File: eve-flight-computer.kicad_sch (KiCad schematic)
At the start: 0 parts

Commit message: Rev. 1
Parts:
- added BT1: ML414H, kicad-egglib:ML414H, symbol Device:Battery_Cell
- added C1, C26: 4.7uF, kicad-egglib:0402_1005M, symbol Device:C_Small
- added C10, C11, C12, C13, C14, C15, C17, C2, C21, C22, C23, C24, C25, C27, C28, C29, C3, C30, C31, C33, C34, C36, C37, C4, C42, C5, C54, C6, C7, C8, C9: 100nF, kicad-egglib:0402_1005M, symbol Device:C_Small
- added C16, C18: 2.2uF, kicad-egglib:0402_1005M, symbol Device:C_Small
- added C19, C32, C35, C43, C44, C45: 10uF, kicad-egglib:0805_2012M, symbol Device:C_Small
- added C20, C38, C39, C40, C41, C46, C47, C48, C49, C50, C51: 47uF, Capacitor_SMD:C_1206_3216Metric, symbol Device:C_Small
- added C52, C53: 22uF, kicad-egglib:0805_2012M, symbol Device:C_Small
- added D1: Red, Diode_SMD:D_0603_1608Metric, symbol Device:LED_Small
- added D10, D11, D6, D9: 11V, Diode_SMD:D_SOD-123, symbol Device:D_Zener_Small
- added D2: Green, Diode_SMD:D_0603_1608Metric, symbol Device:LED_Small
- added D3: Blue, Diode_SMD:D_0603_1608Metric, symbol Device:LED_Small
- added D4: Yellow, Diode_SMD:D_0603_1608Metric, symbol Device:LED_Small
- added D5: PMEG4005EJ, Diode_SMD:D_SOD-323, symbol Device:D_Small
- added D7, D8: UPS115UE3, Diode_SMD:D_Powermite_AK, symbol Device:D_Small
- added J1: USB4110, Connector_USB:USB_C_Receptacle_GCT_USB4110, symbol kicad-egglib:USB-C-2
- added J10, J11, J13, J14, J8, J9: SERVO, Connector_PinHeader_2.54mm:PinHeader_1x03_P2.54mm_Vertical, symbol Connector:Conn_01x03_Pin
- added J12: PYRO, Connector_PinSocket_2.54mm:PinSocket_1x12_P2.54mm_Vertical, symbol Connector:Conn_01x12_Socket
- added J2: ARM Cortex Debug, Connector_PinHeader_1.27mm:PinHeader_2x05_P1.27mm_Vertical_SMD, symbol kicad-egglib:ARM_Cortex_Debug
- added J3: GPIO, Connector_PinSocket_2.54mm:PinSocket_1x12_P2.54mm_Vertical, symbol Connector:Conn_01x12_Socket
- added J4, J5, J6: SMA, Connector_Coaxial:SMA_Amphenol_132289_EdgeMount, symbol Connector:Conn_Coaxial
- added J7: XT-60, kicad-egglib:XT60PW-M, symbol Connector:Conn_01x02_Socket
- added JP1: VSEL, Jumper:SolderJumper-3_P1.3mm_Open_Pad1.0x1.5mm, symbol Jumper:SolderJumper_3_Open
- added L1: 4.7uH, Inductor_SMD:L_1210_3225Metric, symbol Device:L_Small
- added Q1, Q10, Q2, Q3, Q4, Q5, Q6, Q7, Q8: DMG3402L, Package_TO_SOT_SMD:SOT-23-3, symbol Device:Q_NMOS_GSD
- added Q11, Q9: DMP3099L, Package_TO_SOT_SMD:SOT-23-3, symbol Device:Q_PMOS_GSD
- added R1, R2: 5.1k, kicad-egglib:0402_1005M, symbol Device:R_Small_US
- added R10, R30: 3.3k, kicad-egglib:0402_1005M, symbol Device:R_Small_US
- added R11, R12, R13, R14, R15, R16, R17, R20, R4: 100k, kicad-egglib:0402_1005M, symbol Device:R_Small_US
- added R18, R19, R22, R27, R28, R29, R34, R38, R6, R7, R8, R9: 1k, kicad-egglib:0402_1005M, symbol Device:R_Small_US
- added R21, R23, R24, R25, R26, R31, R32, R33, R35, R36, R37, R39, R40, R41, R42, R43, R44: 10k, kicad-egglib:0402_1005M, symbol Device:R_Small_US
- added R3: 33k, kicad-egglib:0402_1005M, symbol Device:R_Small_US
- added R5: 82k, kicad-egglib:0402_1005M, symbol Device:R_Small_US
- added U1: USBLC6-2SC6, Package_TO_SOT_SMD:SOT-23-6, symbol kicad-egglib:USBLC6-2SC6
- added U10: MLX90395KDC, Package_SO:SOIC-8_3.9x4.9mm_P1.27mm, symbol kicad-egglib:MLX90395KDC
- added U11, U8: W25N01GVZEIG, Package_SON:WSON-8-1EP_8x6mm_P1.27mm_EP3.4x4.3mm, symbol kicad-egglib:W25N01GVZEIx
- added U12: LDL1117, Package_TO_SOT_SMD:SOT-223-3_TabPin2, symbol kicad-egglib:Generic_Regulator_GroundOutputInput
- added U13: AP62200WU, Package_TO_SOT_SMD:SOT-23-6, symbol kicad-egglib:AP62200WU
- added U14: INA260, Package_SO:TSSOP-16_4.4x5mm_P0.65mm, symbol kicad-egglib:INA260
- added U15, U16, U17, U18, U19, U20: SN74LVC1T45DBV, Package_TO_SOT_SMD:SOT-23-6, symbol kicad-egglib:SN74LVC1T45DBV
- added U2: STM32H733ZGT6, Package_QFP:LQFP-144_20x20mm_P0.5mm, symbol kicad-egglib:STM32F765ZxTx
- added U3: BMI088, kicad-egglib:BMI088, symbol kicad-egglib:BMI088
- added U4: H3LIS331DL, Package_LGA:LGA-16_3x3mm_P0.5mm_LayoutBorder3x5y, symbol kicad-egglib:H3LIS331DL
- added U5: RFM95W-915S2, kicad-egglib:RFM9xW-xxxS2, symbol kicad-egglib:RFM9xW-xxxS2
- added U6: ZOE-M8Q, kicad-egglib:ZOE-M8Q, symbol kicad-egglib:ZOE-M8Q
- added U7: MS560702BA03-50, kicad-egglib:MS5607-02BA, symbol kicad-egglib:MS5607-02BA
- added U9: RFM96W-433S2, kicad-egglib:RFM9xW-xxxS2, symbol kicad-egglib:RFM9xW-xxxS2
- added Y1: 48MHz, Crystal:Crystal_SMD_2520-4Pin_2.5x2.0mm, symbol Device:Crystal_GND24_Small
- added Y2: 32.768kHz, Crystal:Crystal_SMD_MicroCrystal_CM9V-T1A-2Pin_1.6x1.0mm, symbol Device:Crystal_Small
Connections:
- new net: J12.4 (Pin_4), Q4.3 (D), R27.1
- new net: D9.1 (K), Q3.1 (G), R27.2, R31.1
- new net: C42.2, L1.1, U13.2 (SW)
- new net: C45.1, D7.1 (K), D8.1 (K), U13.3 (VIN)
- new net: R26.2, R30.1, U13.4 (FB)
- new net: C42.1, U13.6 (BST)
- new net: D11.1 (K), Q7.1 (G), R38.2, R39.1
- new net: C44.1, JP1.1 (A), U12.2 (VOUT)
- new net: J12.11 (Pin_11), J7.1 (Pin_1), U14.1 (IN+), U14.12 (VBUS), U14.2 (IN+), U14.3 (IN+)
- new net: J1.A5 (CC1), R2.1
- new net: J12.8 (Pin_8), Q8.3 (D), R38.1
- new net: D6.1 (K), Q1.1 (G), R22.2, R23.1
- new net: J4.1 (In), U6.A4 (RF_IN)
- new net: BT1.1 (+), C25.1, C26.1, R10.1, U6.H9 (V_BCKP)
- new net: U6.J7 (RTC_I), Y2.2
- new net: U6.J8 (RTC_O), Y2.1
- new net: J12.6 (Pin_6), Q6.3 (D), R34.1
- new net: J9.3 (Pin_3), U16.4 (B)
- new net: J6.1 (In), U9.9 (ANT)
- new net: J1.A7 (D-), J1.B7 (D-), U1.4
- new net: J1.A6 (D+), J1.B6 (D+), U1.6
- new net: D10.1 (K), Q5.1 (G), R34.2, R35.1
- new net: Q10.1 (G), Q11.3 (D), R42.1
- new net: J13.3 (Pin_3), U19.4 (B)
- new net: JP1.2 (C), U15.6 (VCCB), U16.6 (VCCB), U17.6 (VCCB), U18.6 (VCCB), U19.6 (VCCB), U20.6 (VCCB)
- new net: D4.2 (A), R9.2
- new net: U2.23 (PH0), Y1.3
- new net: R3.2, R5.1, U2.101 (PA9)
- new net: J1.B5 (CC2), R1.1
- new net: C16.1, U2.71 (VCAP1)
- new net: C18.1, U2.106 (VCAP2)
- new net: J14.3 (Pin_3), U20.4 (B)
- new net: J5.1 (In), U5.9 (ANT)
- new net: Q10.3 (D), Q9.1 (G), R40.2
- new net: D3.2 (A), R8.2
- new net: D2.2 (A), R7.2
- new net: J11.3 (Pin_3), U18.4 (B)
- new net: J12.2 (Pin_2), Q2.3 (D), R22.1
- new net: J8.3 (Pin_3), U15.4 (B)
- new net: D1.2 (A), R6.2
- new net: D5.1 (K), R10.2
- new net: J10.3 (Pin_3), U17.4 (B)
- new net +3.3V: C1.1, C10.1, C11.1, C12.1, C13.1, C14.1, C15.1, C19.1, C2.1, C21.1, C22.1, C23.1, C24.1, C27.1, C28.1, C29.1, C3.1, C30.1, C31.1, C32.1, C33.1, C34.1, C35.1, C36.1, C37.1, C4.1, C5.1, C52.1, C53.1, C6.1, C7.1, C8.1, C9.1, D5.2 (A), J12.9 (Pin_9), J2.1 (VCC), J3.3 (Pin_3), JP1.3 (B), L1.2, R11.1, R12.1, R13.1, R14.1, R15.1, R16.1, R17.1, R18.1, R19.1, R20.1, R21.1, R25.1, R26.1, R28.2, R29.2, R33.1, R37.1, R4.1, U10.7 (VDD), U10.8 (PS/~{CS}), U11.3 (~{WP}/IO2), U11.7 (~{HOLD}/IO3), U11.8 (VCC), U14.10 (VDD), U15.1 (VCCA), U15.5 (DIR), U16.1 (VCCA), U16.5 (DIR), U17.1 (VCCA), U17.5 (DIR), U18.1 (VCCA), U18.5 (DIR), U19.1 (VCCA), U19.5 (DIR), U2.108 (VDD), U2.121 (VDDSDMMC), U2.131 (VDD), U2.143 (PDR_ON), U2.144 (VDD), U2.17 (VDD), U2.30 (VDD), U2.32 (VREF+), U2.33 (VDDA), U2.39 (VDD), U2.52 (VDD), U2.6 (VBAT), U2.62 (VDD), U2.72 (VDD), U2.84 (VDD), U2.95 (VDD), U20.1 (VCCA), U20.5 (DIR), U3.11 (VDDIO), U3.3 (VDD), U4.1 (VDDIO), U4.14 (VDD), U4.15 (VDD), U5.13 (3.3V), U6.G1 (V_CORE), U6.H1 (V_DCDC_OUT), U6.J1 (VCC), U6.J2 (VCC), U7.1 (VDD), U8.3 (~{WP}/IO2), U8.7 (~{HOLD}/IO3), U8.8 (VCC), U9.13 (3.3V), Y1.2
- new net +BATT: C20.1, C43.1, C46.1, C47.1, C48.1, C49.1, C50.1, C51.1, D8.2 (A), J10.2 (Pin_2), J11.2 (Pin_2), J13.2 (Pin_2), J14.2 (Pin_2), J3.1 (Pin_1), J8.2 (Pin_2), J9.2 (Pin_2), Q9.2 (S), R40.1, U12.3 (VIN), U14.14 (IN-), U14.15 (IN-), U14.16 (IN-)
- new net +VSW: C38.1, C39.1, C40.1, C41.1, J12.1 (Pin_1), J12.3 (Pin_3), J12.5 (Pin_5), J12.7 (Pin_7), Q9.3 (D), R43.1
- new net ACC_INT: U2.60 (PE9), U3.16 (INT1)
- new net ACC_~{CS}: R12.2, U2.59 (PE8), U3.14 (~{CS1})
- new net ALT_MISO: U2.112 (PC11), U7.6 (SDO)
- new net ALT_MOSI: U2.113 (PC12), U7.7 (SDA/SDI)
- new net ALT_SCK: U2.111 (PC10), U7.8 (SCL/SCK)
- new net ALT_~{CS}: R15.2, U2.110 (PA15), U7.5 (SA0/~{CS})
- new net COM0_D0: U2.40 (PA4), U5.14 (DIO0)
- new net COM0_D1: U2.37 (PA3), U5.15 (DIO1)
- new net COM0_~{CS}: R14.2, U2.44 (PC4), U5.5 (~{CS})
- new net COM0_~{RST}: U2.45 (PC5), U5.6 (~{RST})
- new net COM1_D0: U2.47 (PB1), U9.14 (DIO0)
- new net COM1_D1: U2.46 (PB0), U9.15 (DIO1)
- new net COM1_~{CS}: R17.2, U2.48 (PB2), U9.5 (~{CS})
- new net COM1_~{RST}: U2.49 (PF11), U9.6 (~{RST})
- new net COM_MISO: U2.42 (PA6), U5.2 (SDO), U9.2 (SDO)
- new net COM_MOSI: U2.43 (PA7), U5.3 (SDI), U9.3 (SDI)
- new net COM_SCK: U2.41 (PA5), U5.4 (SCK), U9.4 (SCK)
- new net GND: BT1.2 (-), C1.2, C10.2, C11.2, C12.2, C13.2, C14.2, C15.2, C16.2, C17.2, C18.2, C19.2, C2.2, C20.2, C21.2, C22.2, C23.2, C24.2, C25.2, C26.2, C27.2, C28.2, C29.2, C3.2, C30.2, C31.2, C32.2, C33.2, C34.2, C35.2, C36.2, C37.2, C38.2, C39.2, C4.2, C40.2, C41.2, C43.2, C44.2, C45.2, C46.2, C47.2, C48.2, C49.2, C5.2, C50.2, C51.2, C52.2, C53.2, C54.2, C6.2, C7.2, C8.2, C9.2, D1.1 (K), D10.2 (A), D11.2 (A), D2.1 (K), D3.1 (K), D4.1 (K), D6.2 (A), D9.2 (A), J1.A1 (GND), J1.A12 (GND), J1.B1 (GND), J1.B12 (GND), J10.1 (Pin_1), J11.1 (Pin_1), J12.12 (Pin_12), J13.1 (Pin_1), J14.1 (Pin_1), J2.3 (GND), J2.5 (GND), J2.9 (GND_Det), J3.12 (Pin_12), J3.2 (Pin_2), J4.2 (Ext), J5.2 (Ext), J6.2 (Ext), J7.2 (Pin_2), J8.1 (Pin_1), J9.1 (Pin_1), Q1.2 (S), Q10.2 (S), Q2.2 (S), Q3.2 (S), Q4.2 (S), Q5.2 (S), Q6.2 (S), Q7.2 (S), Q8.2 (S), R1.2, R2.2, R23.2, R24.2, R30.2, R31.2, R32.2, R35.2, R36.2, R39.2, R41.2, R42.2, R43.2, R44.2, R5.2, U1.2, U10.3 (SDO), U10.5 (SA0), U10.6 (VSS), U11.4 (GND), U12.1 (GND), U13.1 (GND), U14.11 (GND), U14.4 (A1), U14.5 (A0), U14.6 (GND), U15.2 (GND), U16.2 (GND), U17.2 (GND), U18.2 (GND), U19.2 (GND), U2.107 (VSS), U2.120 (VSS), U2.130 (VSS), U2.138 (BOOT0), U2.16 (VSS), U2.31 (VSSA), U2.38 (VSS), U2.51 (VSS), U2.61 (VSS), U2.83 (VSS), U2.94 (VSS), U20.2 (GND), U3.4 (VSSA), U3.6 (VSSIO), U3.7 (PS), U4.10 (GND), U4.12 (GND), U4.13 (GND), U4.16 (GND), U4.5 (GND), U5.1 (GND), U5.10 (GND), U5.8 (GND), U6.A1 (GND), U6.A3 (GND), U6.A5 (GND), U6.A7 (GND), U6.A8 (GND), U6.A9 (GND), U6.B9 (GND), U6.C7 (GND), U6.C9 (GND), U6.D6 (GND), U6.D9 (GND), U6.E7 (GND), U6.F7 (GND), U6.G3 (GND), U6.G6 (GND), U6.G7 (GND), U6.J3 (GND), U6.J9 (GND), U7.2 (PS), U7.3 (GND), U8.4 (GND), U9.1 (GND), U9.10 (GND), U9.8 (GND), Y1.4
- new net GNSS_RX: U2.136 (PB6), U6.J4 (RX/SDI)
- new net GNSS_TX: U2.137 (PB7), U6.J5 (TX/SDO)
- new net GYR_INT: U2.63 (PE10), U3.12 (INT3)
- new net GYR_~{CS}: R13.2, U2.64 (PE11), U3.5 (~{CS2})
- new net HGAC_MISO: U2.75 (PB14), U4.7 (SA0/SDO)
- new net HGAC_MOSI: U2.76 (PB15), U4.6 (SDA/SDI)
- new net HGAC_SCK: U2.74 (PB13), U4.4 (SCL/SCK)
- new net HGAC_~{CS}: R11.2, U2.73 (PB12), U4.8 (~{CS})
- new net IMU_MISO: U2.66 (PE13), U3.10 (SA0/SDO2), U3.15 (SA0/SDO1)
- new net IMU_MOSI: U2.67 (PE14), U3.9 (SDA/SDI)
- new net IMU_SCK: U2.65 (PE12), U3.8 (SCL/SCK)
- new net IO0: J3.4 (Pin_4), U2.114 (PD0)
- new net IO1: J3.5 (Pin_5), U2.115 (PD1)
- new net IO2: J3.6 (Pin_6), U2.116 (PD2)
- new net IO3: J3.7 (Pin_7), U2.117 (PD3)
- new net IO4: J3.8 (Pin_8), U2.118 (PD4)
- new net IO5: J3.9 (Pin_9), U2.119 (PD5)
- new net IO6: J3.10 (Pin_10), U2.122 (PD6)
- new net IO7: J3.11 (Pin_11), U2.123 (PD7)
- new net LED_BLUE: R8.1, U2.79 (PD10)
- new net LED_GREEN: R7.1, U2.78 (PD9)
- new net LED_RED: R6.1, U2.77 (PD8)
- new net LED_YELLOW: R9.1, U2.80 (PD11)
- new net MAG_INT: U10.4 (INT/TRIG), U2.12 (PF2)
- new net MAG_SCL: R18.2, U10.1 (SCL/SCK), U2.11 (PF1)
- new net MAG_SDA: R19.2, U10.2 (SDA/SDI), U2.10 (PF0)
- new net MCU_SWCLK: J2.4 (SWCLK/TCK), U2.109 (PA14)
- new net MCU_SWDIO: J2.2 (SWDIO/TMS), U2.105 (PA13)
- new net MCU_~{RST}: C17.1, J2.10 (~{RST}), R4.2, U2.25 (~{RST})
- new net MEM0_~{CS}: R16.2, U2.125 (PG10), U8.1 (~{CS})
- new net MEM1_~{CS}: R20.2, U11.1 (~{CS}), U2.126 (PG11)
- new net MEM_MISO: U11.2 (SDO/IO1), U2.127 (PG12), U8.2 (SDO/IO1)
- new net MEM_MOSI: U11.5 (SDI/IO0), U2.129 (PG14), U8.5 (SDI/IO0)
- new net MEM_SCK: U11.6 (SCK), U2.128 (PG13), U8.6 (SCK)
- new net PWR_SCL: R29.1, U14.9 (SCL), U2.54 (PF14)
- new net PWR_SDA: R28.1, U14.8 (SDA), U2.55 (PF15)
- new net PYRO0_FIRE: Q2.1 (G), R24.1, U2.14 (PF4)
- new net PYRO0_~{CONT}: Q1.3 (D), R21.2, U2.13 (PF3)
- new net PYRO1_FIRE: Q4.1 (G), R32.1, U2.18 (PF6)
- new net PYRO1_~{CONT}: Q3.3 (D), R25.2, U2.15 (PF5)
- new net PYRO2_FIRE: Q6.1 (G), R36.1, U2.20 (PF8)
- new net PYRO2_~{CONT}: Q5.3 (D), R33.2, U2.19 (PF7)
- new net PYRO3_FIRE: Q8.1 (G), R41.1, U2.22 (PF10)
- new net PYRO3_~{CONT}: Q7.3 (D), R37.2, U2.21 (PF9)
- new net PYRO_EN: Q11.2 (S), U2.36 (PA2)
- new net SERVO0: U15.3 (A), U2.81 (PD12)
- new net SERVO1: U16.3 (A), U2.82 (PD13)
- new net SERVO2: U17.3 (A), U2.85 (PD14)
- new net SERVO3: U18.3 (A), U2.86 (PD15)
- new net SERVO4: U19.3 (A), U2.96 (PC6)
- new net SERVO5: U2.97 (PC7), U20.3 (A)
- new net USB_D+: U1.1, U2.104 (PA12)
- new net USB_D-: U1.3, U2.103 (PA11)
- new net VBUS: D7.2 (A), J1.A4 (VBUS), J1.A9 (VBUS), J1.B4 (VBUS), J1.B9 (VBUS), R3.1, U1.5
- new net ~{ENABLE}: C54.1, J12.10 (Pin_10), Q11.1 (G), R44.1, U2.35 (PA1)
- no-connect marks 0 -> 79
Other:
- note added: "INPUT 18V MAX"
- note added: "PWR"
- note added: "PYRO0"
- note added: "PYRO1"
- note added: "PYRO2"
- note added: "PYRO3"
- note added: "~{ENABLE}"

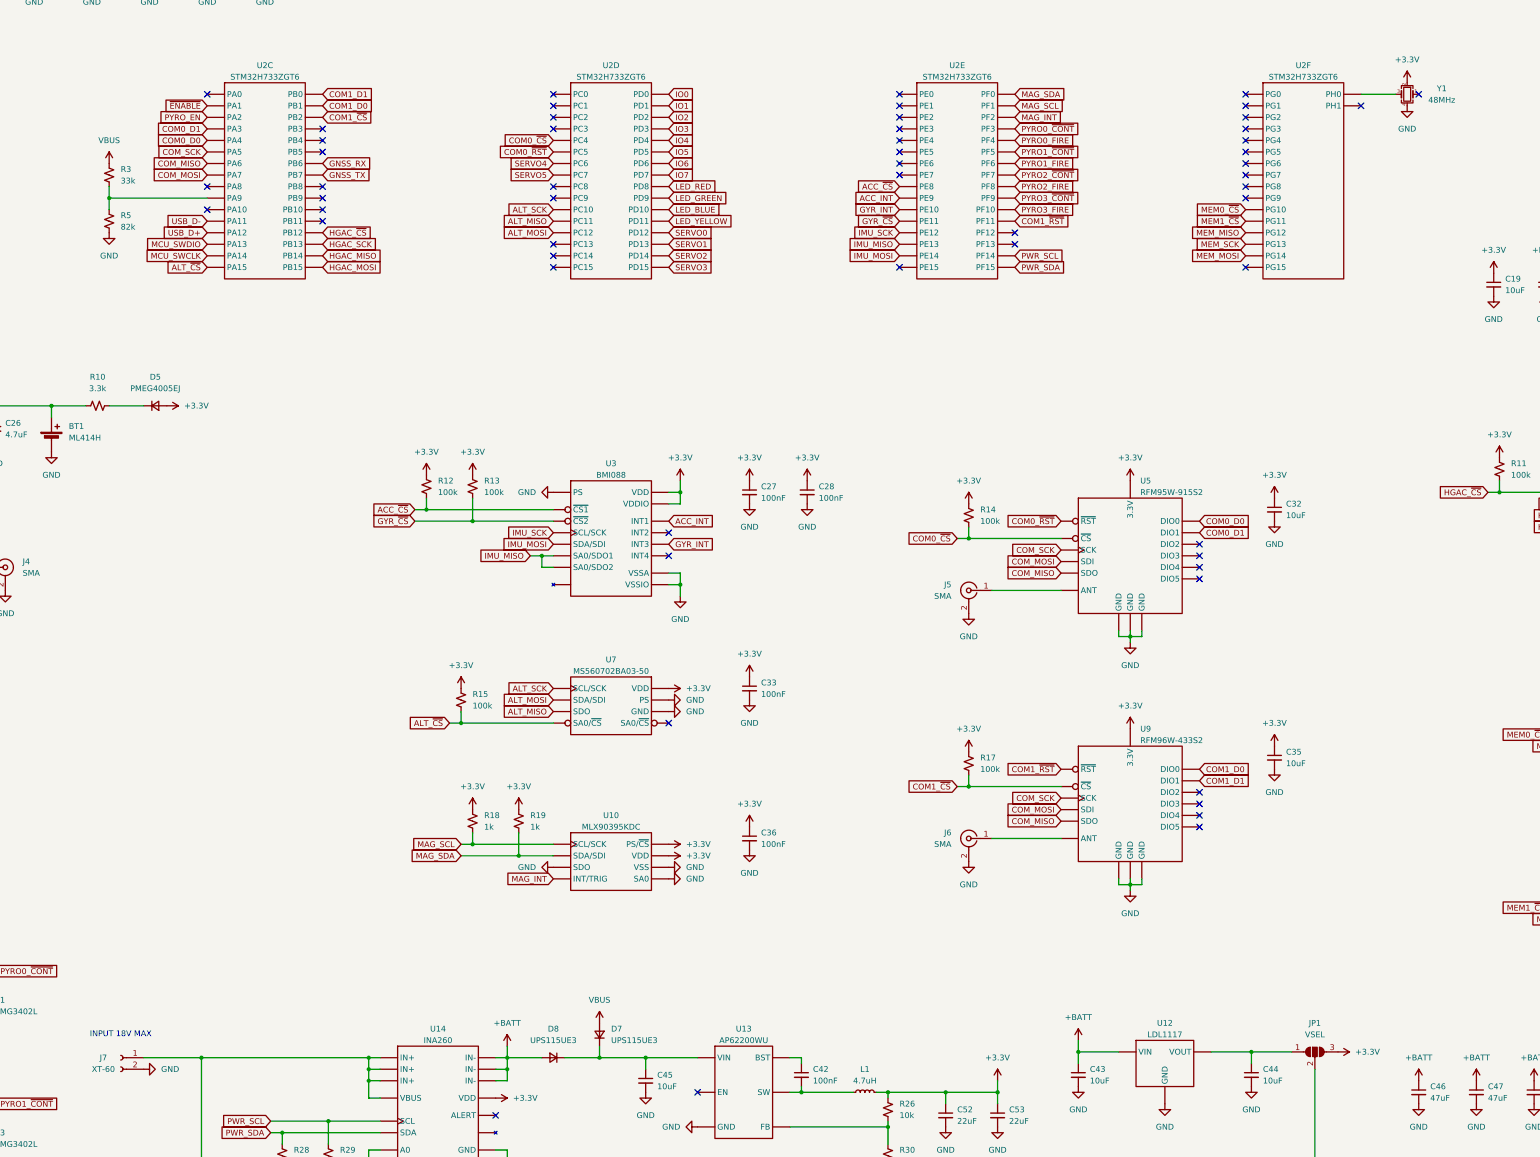
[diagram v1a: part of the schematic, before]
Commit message: Rev. 2
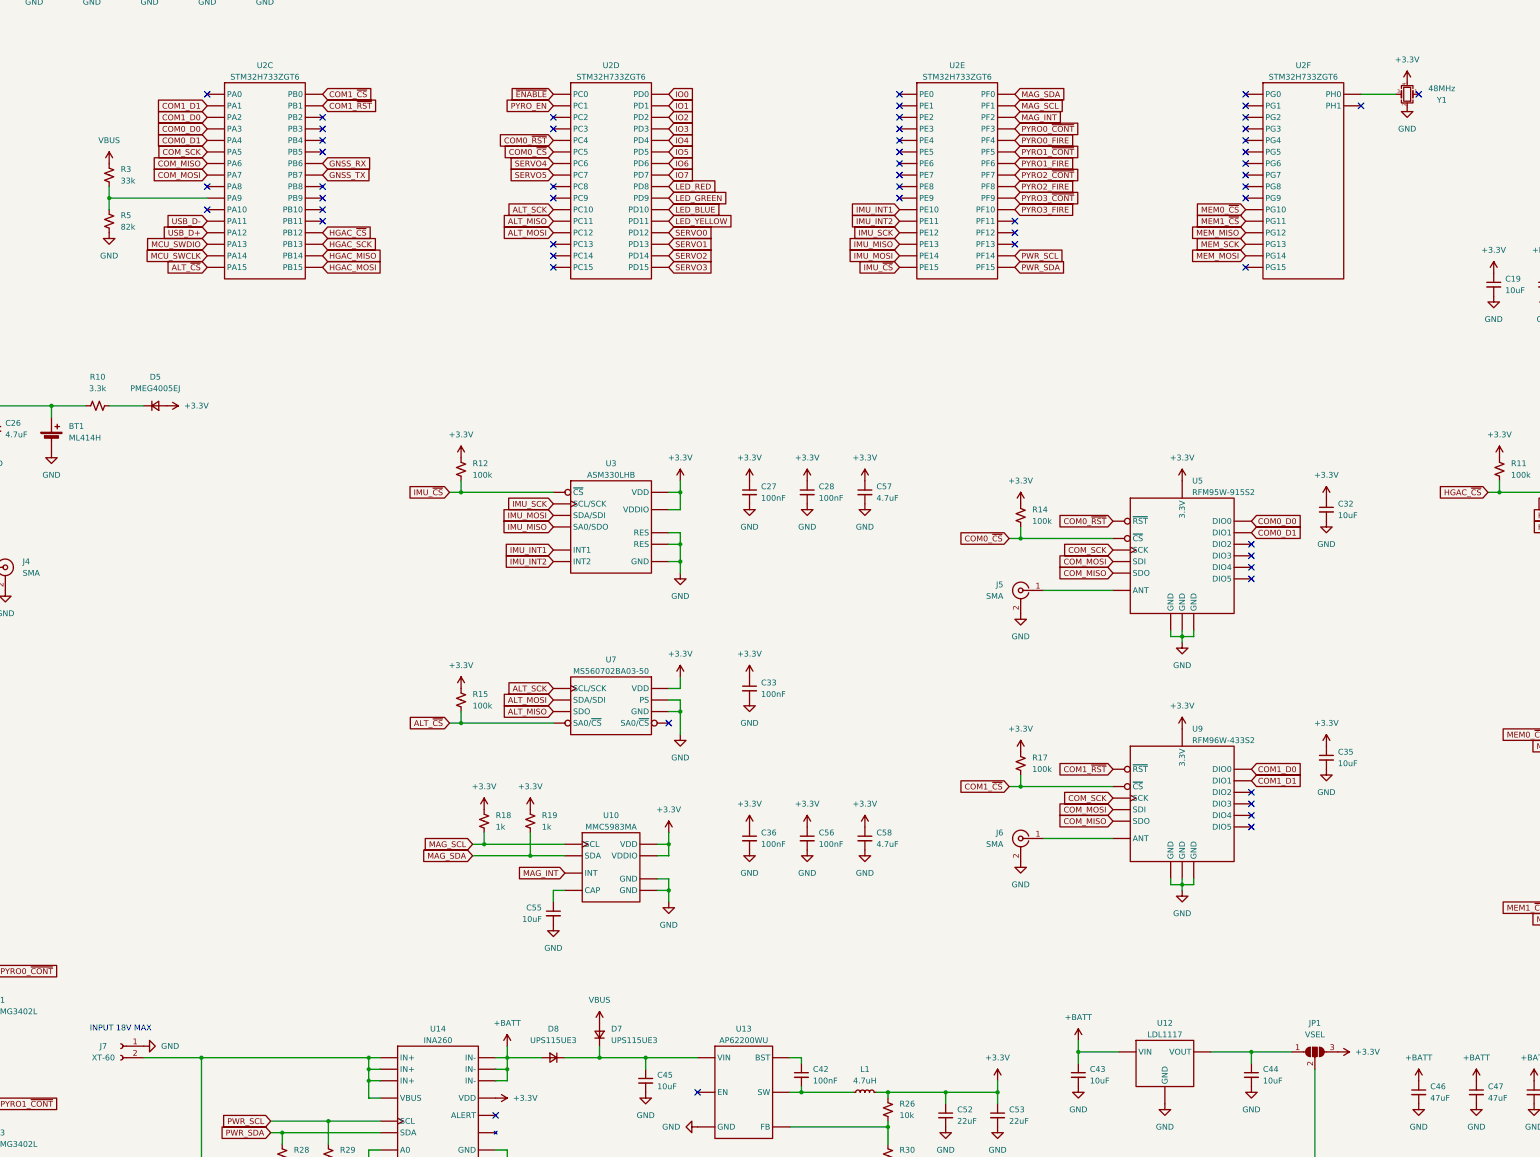
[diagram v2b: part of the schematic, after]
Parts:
- removed R13: 100k, kicad-egglib:0402_1005M, symbol Device:R_Small_US
- removed U10: MLX90395KDC, Package_SO:SOIC-8_3.9x4.9mm_P1.27mm, symbol kicad-egglib:MLX90395KDC
- removed U3: BMI088, kicad-egglib:BMI088, symbol kicad-egglib:BMI088
- added C55: 10uF, kicad-egglib:0805_2012M, symbol Device:C_Small
- added C56: 100nF, kicad-egglib:0402_1005M, symbol Device:C_Small
- added C57, C58: 4.7uF, kicad-egglib:0402_1005M, symbol Device:C_Small
- added U10: MMC5983MA, Package_LGA:LGA-16_3x3mm_P0.5mm, symbol kicad-egglib:MMC5983MA
- added U3: ASM330LHB, Package_LGA:LGA-14_3x2.5mm_P0.5mm_LayoutBorder3x4y, symbol kicad-egglib:ASM330LHB
- BT1: Part # ML414H IV01E -> ML414H-IV01E
- C20, C38, C39, C40, C41, C46, C47, C48, C49, C50, C51: Manufacturer Murata -> Generic; Part # GRM31CR61E476ME44K -> Generic 47uF 25V X5R 1206 MLCC
- D7, D8: Part # UPS115UE3 -> UPS115UE3/TR7
- J1: Part # USB4110 -> USB4110-GF-A
- J10, J11, J13, J14, J8, J9: footprint Connector_PinHeader_2.54mm:PinHeader_1x03_P2.54mm_Vertical -> Connector_JST:JST_XH_B3B-XH-A_1x03_P2.50mm_Vertical; Manufacturer (none) -> JST; Part # (none) -> B3B-XH-A
- Q1, Q10, Q2, Q3, Q4, Q5, Q6, Q7, Q8: Part # DMG3402L -> DMG3402L-7
- Q11, Q9: Part # DMP3099L -> DMP3099L-7
- U14: Part # INA260 -> INA260AIPWR
- U4: Part # H3LIS331DL -> H3LIS331DLTR
- U6: Part # ZOE-M8Q -> ZOE-M8Q-0
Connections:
- net +3.3V: now also Y1.4, C56.1, C57.1, C58.1, U10.13 (VDDIO), U10.2 (VDD), U3.5 (VDDIO), U3.8 (VDD); no longer Y1.2
- net COM0_D0: now also U2.37 (PA3); no longer U2.40 (PA4)
- net COM0_D1: now also U2.40 (PA4); no longer U2.37 (PA3)
- net COM0_~{CS}: now also U2.45 (PC5); no longer U2.44 (PC4)
- net COM0_~{RST}: now also U2.44 (PC4); no longer U2.45 (PC5)
- net COM1_D0: now also U2.36 (PA2); no longer U2.47 (PB1)
- net COM1_D1: now also U2.35 (PA1); no longer U2.46 (PB0)
- net COM1_~{CS}: now also U2.46 (PB0); no longer U2.48 (PB2)
- net COM1_~{RST}: now also U2.47 (PB1); no longer U2.49 (PF11)
- net GND: now also J7.1 (Pin_1), Y1.2, C55.2, C56.2, C57.2, C58.2, U10.11 (GND), U10.9 (GND), U3.2 (RES), U3.3 (RES), U3.7 (GND); no longer J7.2 (Pin_2), Y1.4
- net IMU_MISO: now also U3.1 (SA0/SDO)
- net IMU_MOSI: now also U3.14 (SDA/SDI)
- net IMU_SCK: now also U3.13 (SCL/SCK)
- net MAG_INT: now also U10.15 (INT)
- net MAG_SCL: now also U10.1 (SCL)
- net MAG_SDA: now also U10.16 (SDA)
- net PYRO_EN: now also U2.27 (PC1); no longer U2.36 (PA2)
- net ~{ENABLE}: now also U2.26 (PC0); no longer U2.35 (PA1)
- net at J12.11 (Pin_11), U14.1 (IN+), U14.12 (VBUS)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: now also J7.2 (Pin_2); no longer J7.1 (Pin_1)
- net IMU_~{CS}: now reaches U2.68 (PE15)
- net IMU_~{CS}: now also R12.2, U3.12 (~{CS})
- net ACC_INT: no longer names the net of U2.60 (PE9)
- net ACC_~{CS}: no longer names the net of U2.59 (PE8)
- net ACC_~{CS}: no longer R12.2
- net GYR_INT renamed IMU_INT1
- net IMU_INT1: now also U3.4 (INT1)
- net GYR_~{CS} renamed IMU_INT2
- net IMU_INT2: now also U3.9 (INT2)
- new net: C55.1, U10.10 (CAP)
- new net: U10.12, U10.14, U10.3, U10.4, U10.5, U10.6, U10.7, U10.8
- new net: U3.10, U3.11, U3.6
- no-connect marks 79 -> 78
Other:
- moved on the sheet: C32, C35, J5, J6, J7, R12, R14, R17, R18, R19, U5, U9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
